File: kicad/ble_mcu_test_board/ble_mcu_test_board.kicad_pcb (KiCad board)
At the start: 2 copper layers, 28 parts, among them J1 I2C_MUX_OUT, J2 SWD, SW1 SW_SPDT, SW2 SW_Push, U1 STM32WB10CCUx, U2 DLF162500LT-5028A1, U3 AMS1117-3.3, U4 TCA9548APWR

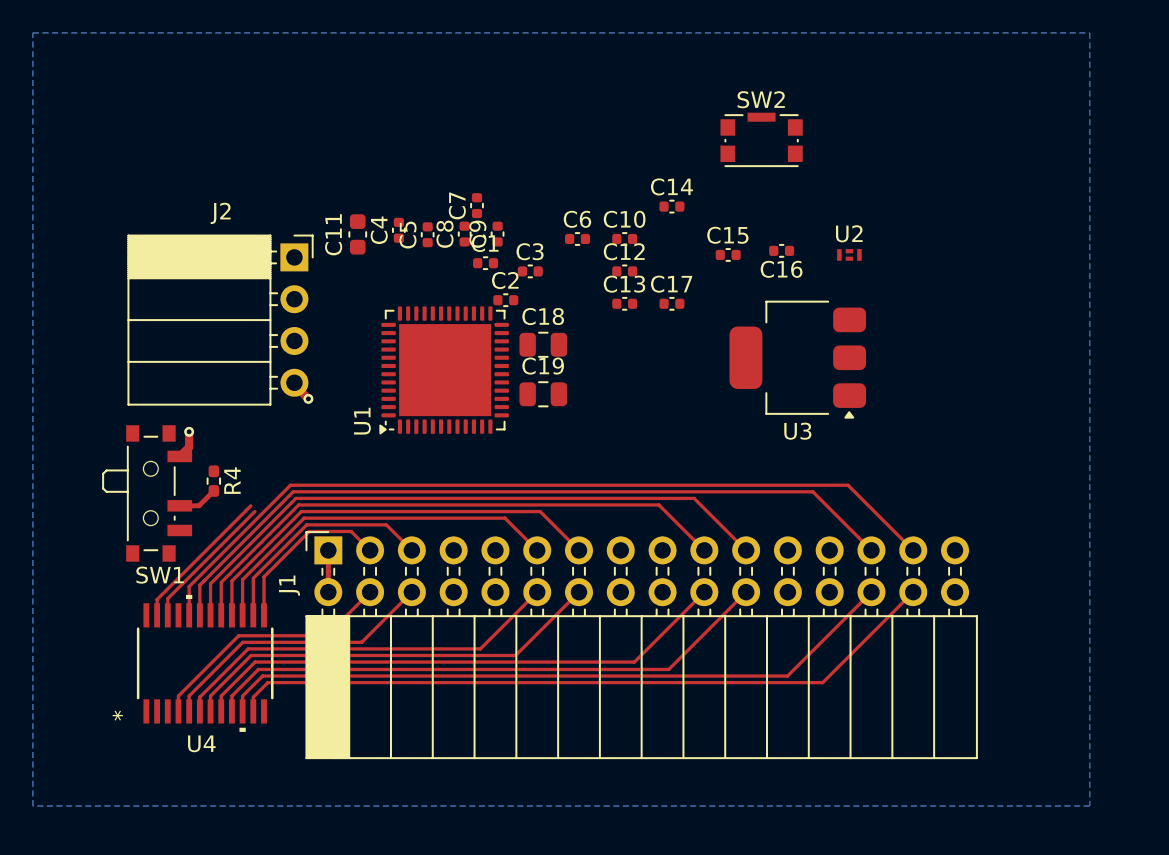
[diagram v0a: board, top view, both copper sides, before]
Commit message: prototype schematic + pcb finalized and ordered
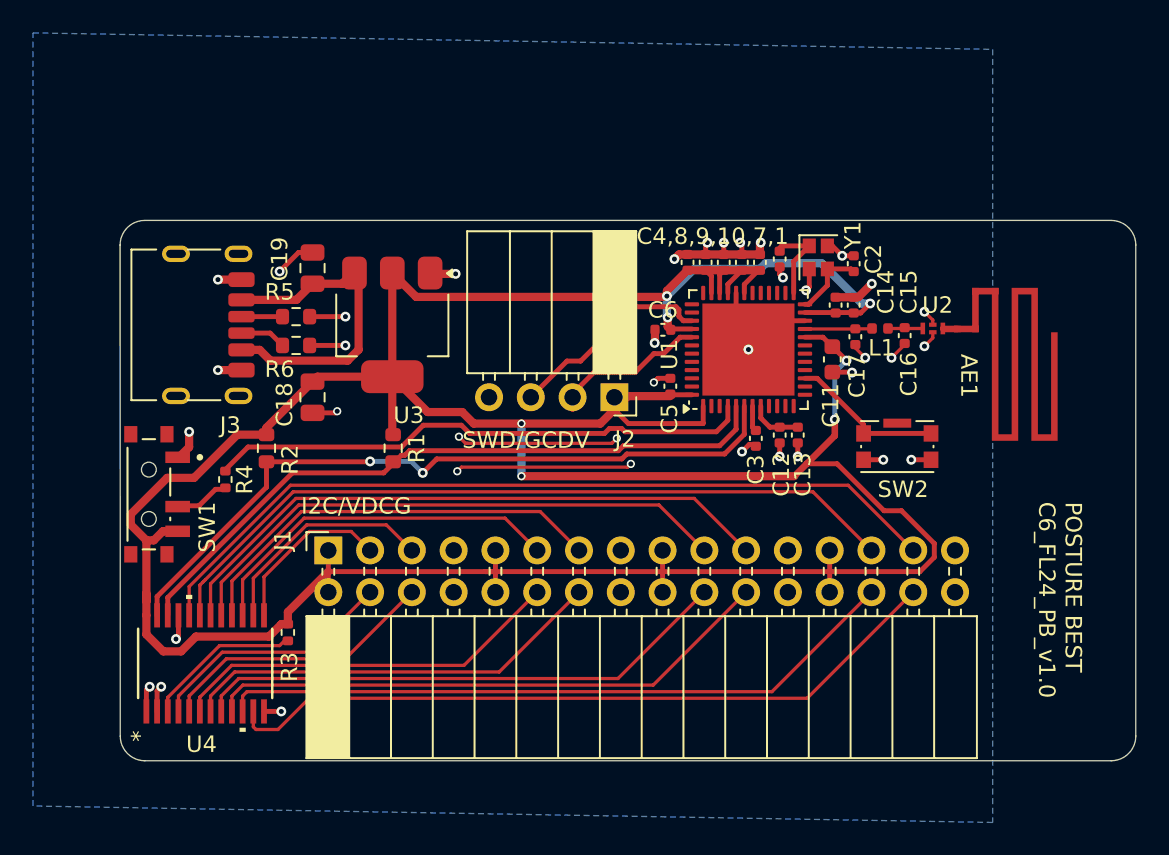
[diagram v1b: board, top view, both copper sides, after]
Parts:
- added AE1: Antenna, pcb_antenna:meander_antenna_stm32wb10cc, F.Cu at (163.0, 85.8)
- added J3: USB_C_Receptacle_PowerOnly_6P, Connector_USB:USB_C_Receptacle_HRO_TYPE-C-31-M-17, F.Cu at (116.5, 85.5)
- added L1: 2.7n, Inductor_SMD:L_0402_1005Metric, F.Cu at (158.5, 85.7)
- added R1: 4k7, Resistor_SMD:R_0603_1608Metric, F.Cu at (128.9, 93.0)
- added R2: 4k7, Resistor_SMD:R_0603_1608Metric, F.Cu at (121.2, 93.0)
- added R3: 4k7, Resistor_SMD:R_0402_1005Metric, F.Cu at (122.5, 104.2)
- added R5: 5k1, Resistor_SMD:R_0603_1608Metric, F.Cu at (123.0, 85.0)
- added R6: 5k1, Resistor_SMD:R_0603_1608Metric, F.Cu at (123.0, 86.8)
- added Y1: 32MHz, Crystal:Crystal_SMD_2016-4Pin_2.0x1.6mm, F.Cu at (154.8, 81.4)
- R4: footprint Resistor_SMD:R_0402_1005Metric_Pad0.72x0.64mm_HandSolder -> Resistor_SMD:R_0402_1005Metric
- SW1: footprint Button_Switch_SMD:SW_SPDT_PCM12 -> external_footprints:SW_SSSS811101
- moved C11 29.8 mm to (155.6, 87.6), turned to -90 degrees
- moved U3 24.7 mm to (128.8, 85.5), turned to -90 degrees
- moved C2 21.3 mm to (156.9, 81.8), turned to 90 degrees
- moved J2 21.2 mm to (142.3, 89.9), turned to -90 degrees
- moved SW2 20.3 mm to (159.6, 92.9)
- moved U1 18.5 mm to (150.5, 87.0)
- moved C1 17.9 mm to (152.4, 81.5), turned to -90 degrees
- moved C4 17.7 mm to (146.8, 81.7)
- moved C7 17.5 mm to (151.2, 81.7)
- moved C5 17.4 mm to (145.8, 89.2)
- moved C3 17.1 mm to (150.9, 92.4), turned to -90 degrees
- moved C19 16.0 mm to (124.0, 82.0), turned to 90 degrees
- moved C8 14.8 mm to (147.9, 81.7)
- moved C18 14.4 mm to (124.0, 89.9), turned to -90 degrees
- moved C9 13.9 mm to (149.0, 81.7)
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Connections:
- U1 pad 39: Net-(J2-Pin_2) -> Net-(J2-Pin_3)
- U1 pad 41: Net-(J2-Pin_3) -> Net-(J2-Pin_2)
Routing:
- net +3.3V: track 2.54 -> 222.8 mm, vias 0 -> 7
- net GND: track 3.07 -> 76.0 mm, vias 2 -> 38
- net Net-(U1-PB9): track 9.02 -> 44.1 mm, vias 0 -> 2
- net BOOT0: track 0.00 -> 33.2 mm
- net Net-(U1-PB8): track 8.51 -> 41.3 mm
- net VBUS: track 0.00 -> 20.2 mm
- net Net-(J2-Pin_3): track 0.00 -> 12.7 mm
- net Net-(J2-Pin_2): track 0.00 -> 9.64 mm
- net Net-(U1-PA6): track 0.00 -> 9.60 mm
- net Net-(U4-*RESET): track 0.00 -> 9.58 mm
- net Net-(U1-OSC_IN): track 0.00 -> 5.11 mm
- net Net-(U1-OSC_OUT): track 0.00 -> 4.51 mm
- net RF_OUT: track 0.00 -> 4.09 mm
- net +3.3VA: track 0.00 -> 3.21 mm
- net Net-(J3-CC2): track 0.00 -> 2.81 mm
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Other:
- board outline added: 61.8 x 32.9 mm
- board text added: "C4,8,9,10,7,1"
- board text added: "I2C/VDCG"
- board text added: "POSTURE BEST C6_FL24_PB_v1.0"
- board text added: "SWD/GCDV"
